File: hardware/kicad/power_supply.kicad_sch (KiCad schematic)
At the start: 29 parts, among them Q1 FZT690B, Q2 FZT790A, U6 TPS60401, U7 ADP7156ARDZ

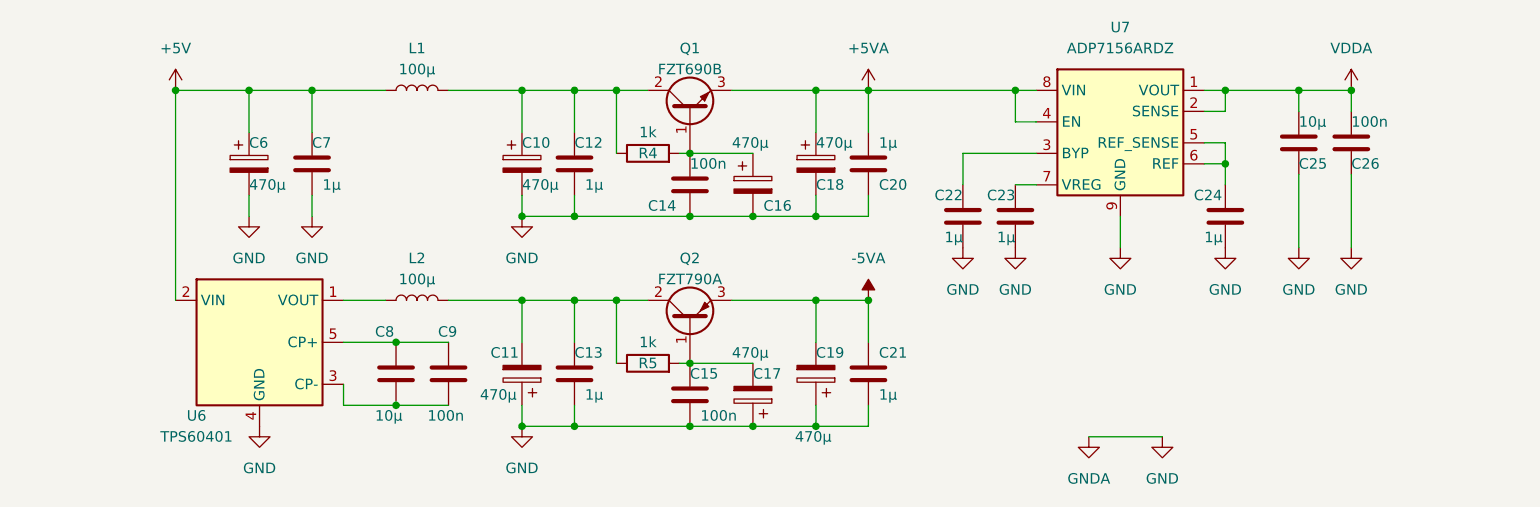
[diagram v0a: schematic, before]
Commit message: new hardware revision
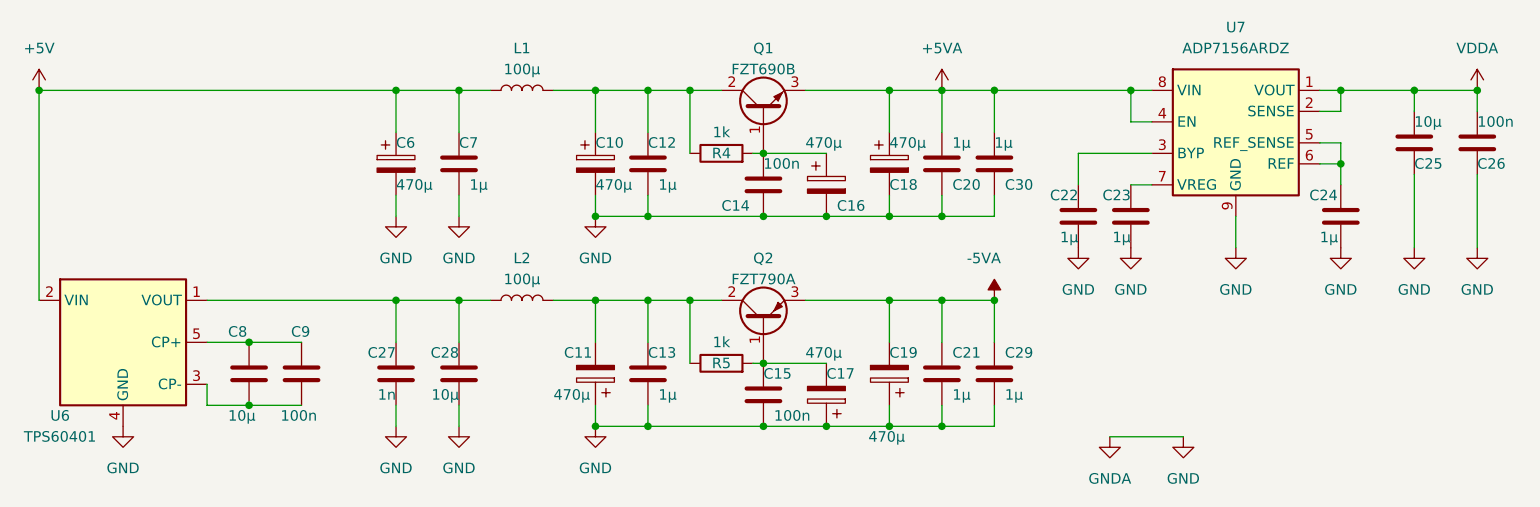
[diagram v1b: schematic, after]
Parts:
- added C27: 1n, Capacitor_SMD:C_0805_2012Metric, symbol Device:C
- added C28: 10µ, Capacitor_SMD:C_0805_2012Metric, symbol Device:C
- added C29, C30: 1µ, Capacitor_SMD:C_0805_2012Metric, symbol Device:C
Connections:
- net +5VA: now also C30.1
- net -5VA: now also C29.1
- net GND: now also C27.1, C28.1, C29.2, C30.2
- net at L2.1, U6.1 (VOUT): now also C27.2, C28.2
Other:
- title: FX3 USB3 ADC -> MISRC
- moved on the sheet: C10, C11, C12, C13, C14, C15, C16, C17, C18, C19, C20, C21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
